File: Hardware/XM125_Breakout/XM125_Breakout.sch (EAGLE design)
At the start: 54 parts, among them J13 SWD (DNP), J2 RIGHT_ANGLE, J3 RIGHT_ANGLE, U1 XM125, U2 RT9080-33GJ5, U3 RT9080-18GJ5, U4 CH340C, U5 ESD Diode

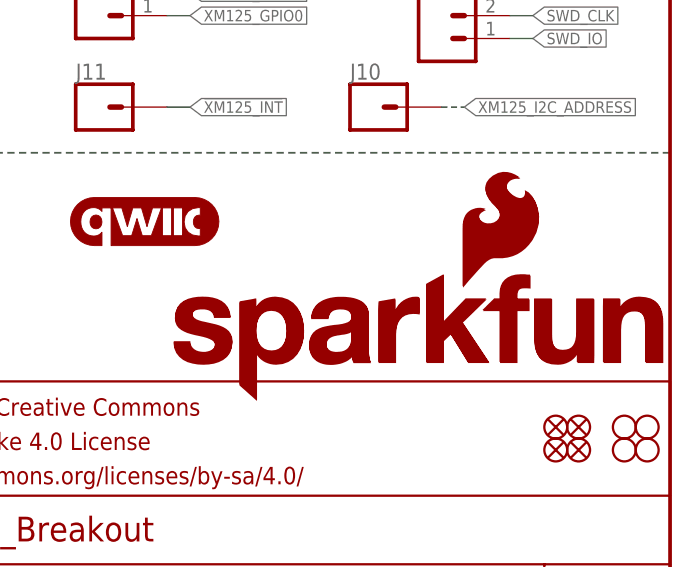
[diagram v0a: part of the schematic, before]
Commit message: Production files added
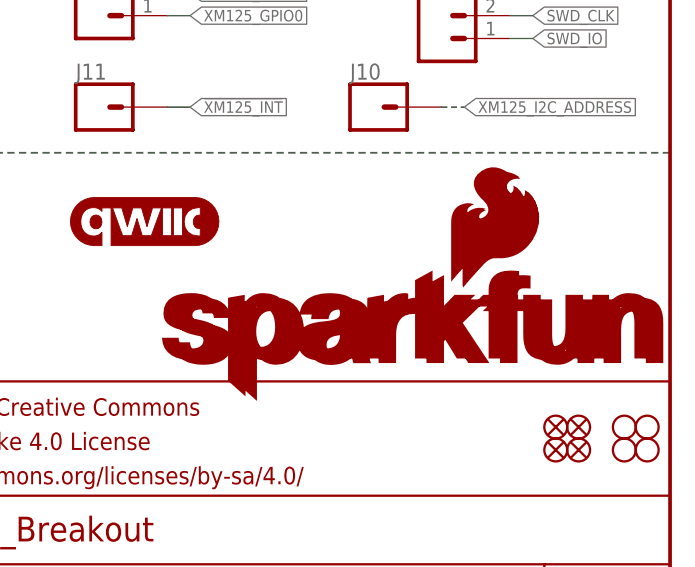
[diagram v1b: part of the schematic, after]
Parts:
- LOGO6: value SFE_LOGO_NAME.1_INCH -> SFE_LOGO_NAME_FLAME.1_INCH; device SparkFun-Aesthetics:SFE_LOGO_NAME.1_INCH -> SparkFun-Aesthetics:SFE_LOGO_NAME_FLAME.1_INCH
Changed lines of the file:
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@@
 <part name="LOGO4" library="SparkFun-Aesthetics" deviceset="OSHW-LOGO" device="S"/>
 <part name="LOGO5" library="SparkFun-Aesthetics" deviceset="SFE_LOGO_FLAME" device=".1_INCH"/>
-<part name="LOGO6" library="SparkFun-Aesthetics" deviceset="SFE_LOGO_NAME" device=".1_INCH"/>
+<part name="LOGO6" library="SparkFun-Aesthetics" deviceset="SFE_LOGO_NAME_FLAME" device=".1_INCH"/>
 <part name="GND1" library="SparkFun-PowerSymbols" deviceset="GND" device=""/>
 <part name="SUPPLY1" library="SparkFun-PowerSymbols" deviceset="1.8V" device=""/>
